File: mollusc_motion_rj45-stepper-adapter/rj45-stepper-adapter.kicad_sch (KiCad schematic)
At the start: 3 parts, among them J2 Conn_01x03, J3 RJ45_Shielded, J6 Conn_01x06

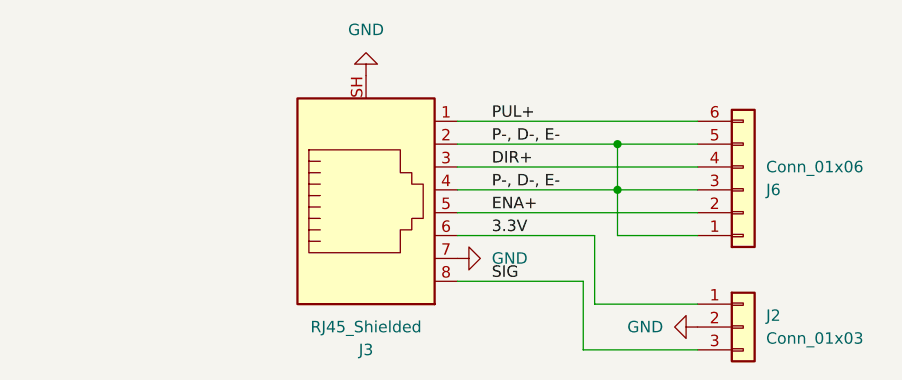
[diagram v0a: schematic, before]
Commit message: v3
in production
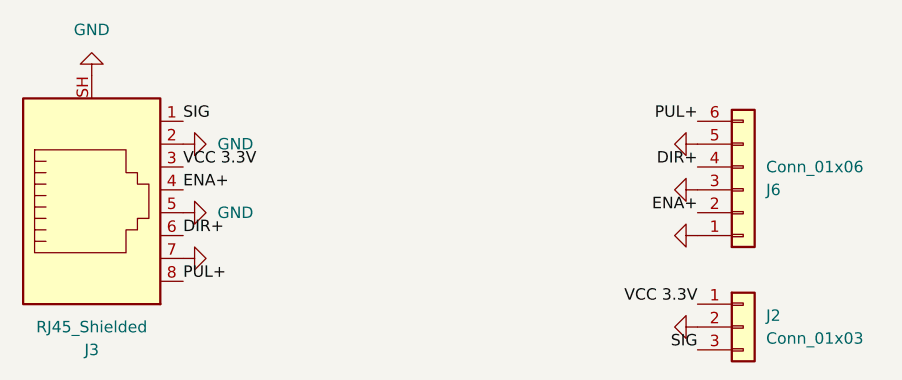
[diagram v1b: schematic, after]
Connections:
- net DIR+: now also J3.6; no longer J3.3
- net ENA+: now also J3.4; no longer J3.5
- net GND: now also J3.2, J3.5, J6.1 (Pin_1), J6.3 (Pin_3), J6.5 (Pin_5)
- net PUL+: now also J3.8; no longer J3.1
- net SIG: now also J3.1; no longer J3.8
- net 3.3V renamed VCC 3.3V
- net VCC 3.3V: now also J3.3; no longer J3.6
- removed net P-, D-, E-: J3.2, J3.4, J6.1 (Pin_1), J6.3 (Pin_3), J6.5 (Pin_5)
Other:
- moved on the sheet: J3
